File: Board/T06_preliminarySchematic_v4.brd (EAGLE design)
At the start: 59.4 x 80 mm, 57 parts, among them M1 SSW-102-02-S-S, M2 SSW-102-02-S-S, Q3 2n3904, U1 ATMEGA328P_PDIP, X1 SSW-105-02-S-S, X2 SSW-102-02-S-S

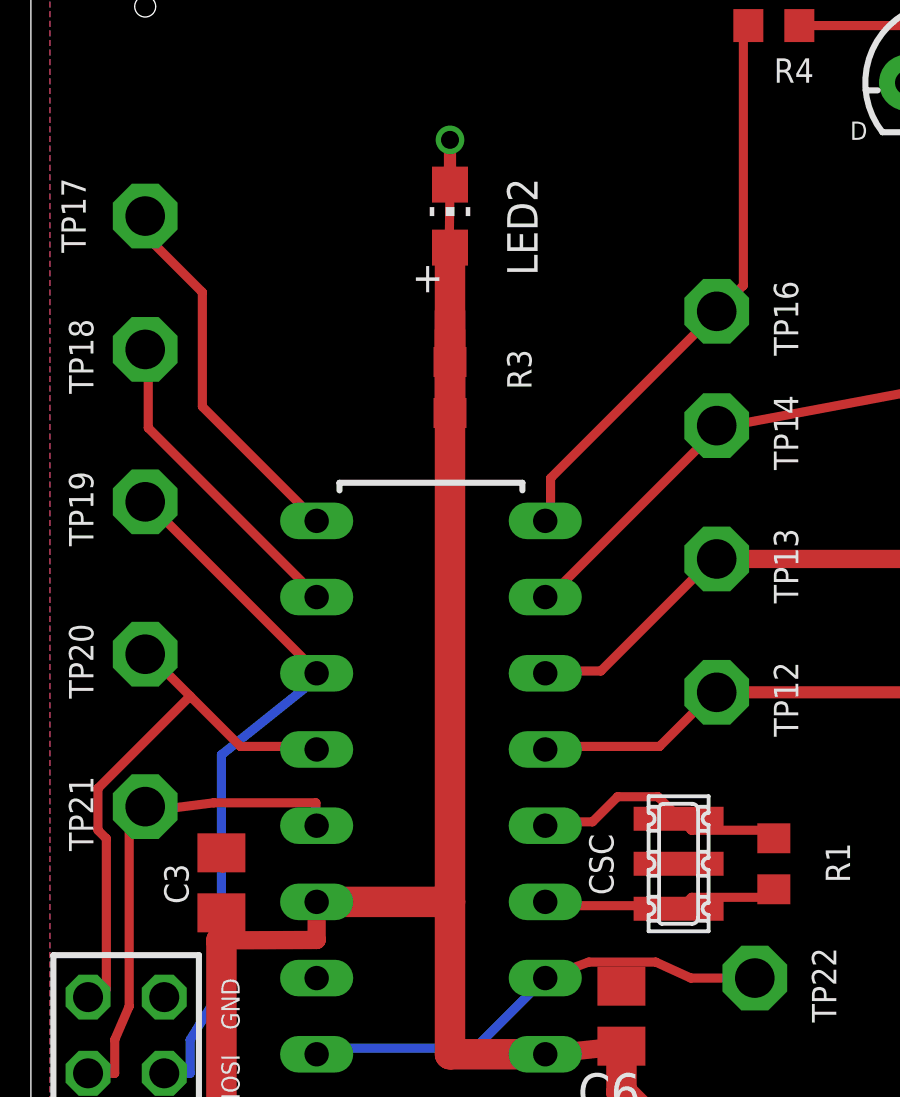
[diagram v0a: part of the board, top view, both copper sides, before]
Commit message: minor adjustments
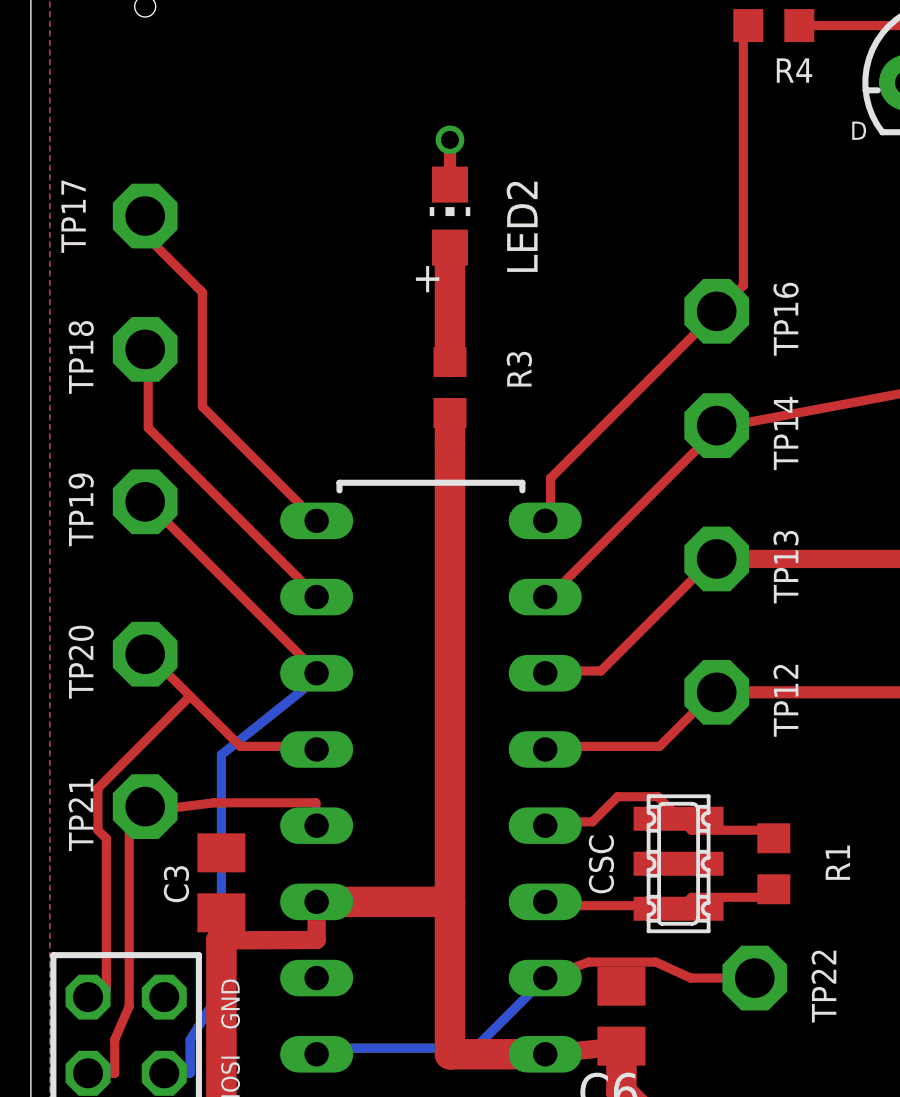
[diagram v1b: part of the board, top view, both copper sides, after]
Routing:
- net +5V: track 175.4 -> 169.2 mm
- net GND: track 58.0 -> 56.0 mm
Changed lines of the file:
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@@
 <?xml version="1.0" encoding="utf-8"?>
 <!DOCTYPE eagle SYSTEM "eagle.dtd">
-<eagle version="7.3.0">
+<eagle version="7.4.0">
 <drawing>
 <settings>
@@
 <layer number="42" name="bRestrict" color="1" fill="10" visible="yes" active="yes"/>
 <layer number="43" name="vRestrict" color="2" fill="10" visible="yes" active="yes"/>
-<layer number="44" name="Drills" color="7" fill="1" visible="no" active="yes"/>
+<layer number="44" name="Drills" color="7" fill="1" visible="yes" active="yes"/>
 <layer number="45" name="Holes" color="7" fill="1" visible="yes" active="yes"/>
 <layer number="46" name="Milling" color="3" fill="1" visible="yes" active="yes"/>
@@
 <wire x1="21.59" y1="48.895" x2="20.3454" y2="48.895" width="0.3048" layer="1"/>
 <wire x1="6.4008" y1="48.7426" x2="6.35" y2="49.26" width="0.3048" layer="1"/>
-<wire x1="13.9446" y1="69.5452" x2="13.97" y2="71.535" width="0.3048" layer="1"/>
 <wire x1="23.8506" y1="45.085" x2="24.384" y2="45.1866" width="0.3048" layer="1"/>
 <wire x1="30.734" y1="22.0726" x2="30.734" y2="17.3228" width="0.3048" layer="1"/>
@@
 <wire x1="6.35" y1="46.3296" x2="6.35" y2="39.37" width="1.016" layer="1"/>
 <wire x1="6.35" y1="39.37" x2="4.445" y2="39.37" width="1.016" layer="1"/>
-<wire x1="13.97" y1="47.625" x2="13.97" y2="67.31" width="1.016" layer="1"/>
-<wire x1="13.97" y1="66.675" x2="13.97" y2="63.92" width="1.016" layer="1"/>
-<wire x1="13.97" y1="67.31" x2="13.97" y2="66.675" width="0" layer="19" extent="1-1"/>
-<wire x1="6.35" y1="46.355" x2="6.35" y2="46.3296" width="0" layer="19" extent="1-1"/>
+<wire x1="13.97" y1="47.625" x2="13.97" y2="62.23" width="1.016" layer="1"/>
+<wire x1="13.97" y1="62.23" x2="13.97" y2="62.865" width="1.016" layer="1"/>
+<wire x1="13.97" y1="62.865" x2="13.97" y2="63.92" width="1.016" layer="1"/>
+<wire x1="6.35" y1="46.3296" x2="6.35" y2="46.355" width="0" layer="19" extent="1-1"/>
 </signal>
 <signal name="N$5">
